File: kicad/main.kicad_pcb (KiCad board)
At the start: 2 copper layers, 119.4 x 99.1 mm, 41 parts, among them J1 Barrel_Jack, SW1 Reset, SW6 SW_DIP_x08, U1 KM1810VM88, U10 L7805, U11 15 MHz, U12 8255, U13 74HC273, U14 74HC244, U2 W27C512, U3 AS6C4008-55PCN, U4 74HC573, U5 74HC573, U6 ATF16V8, U7 DS1813-5+, U8 74HC00

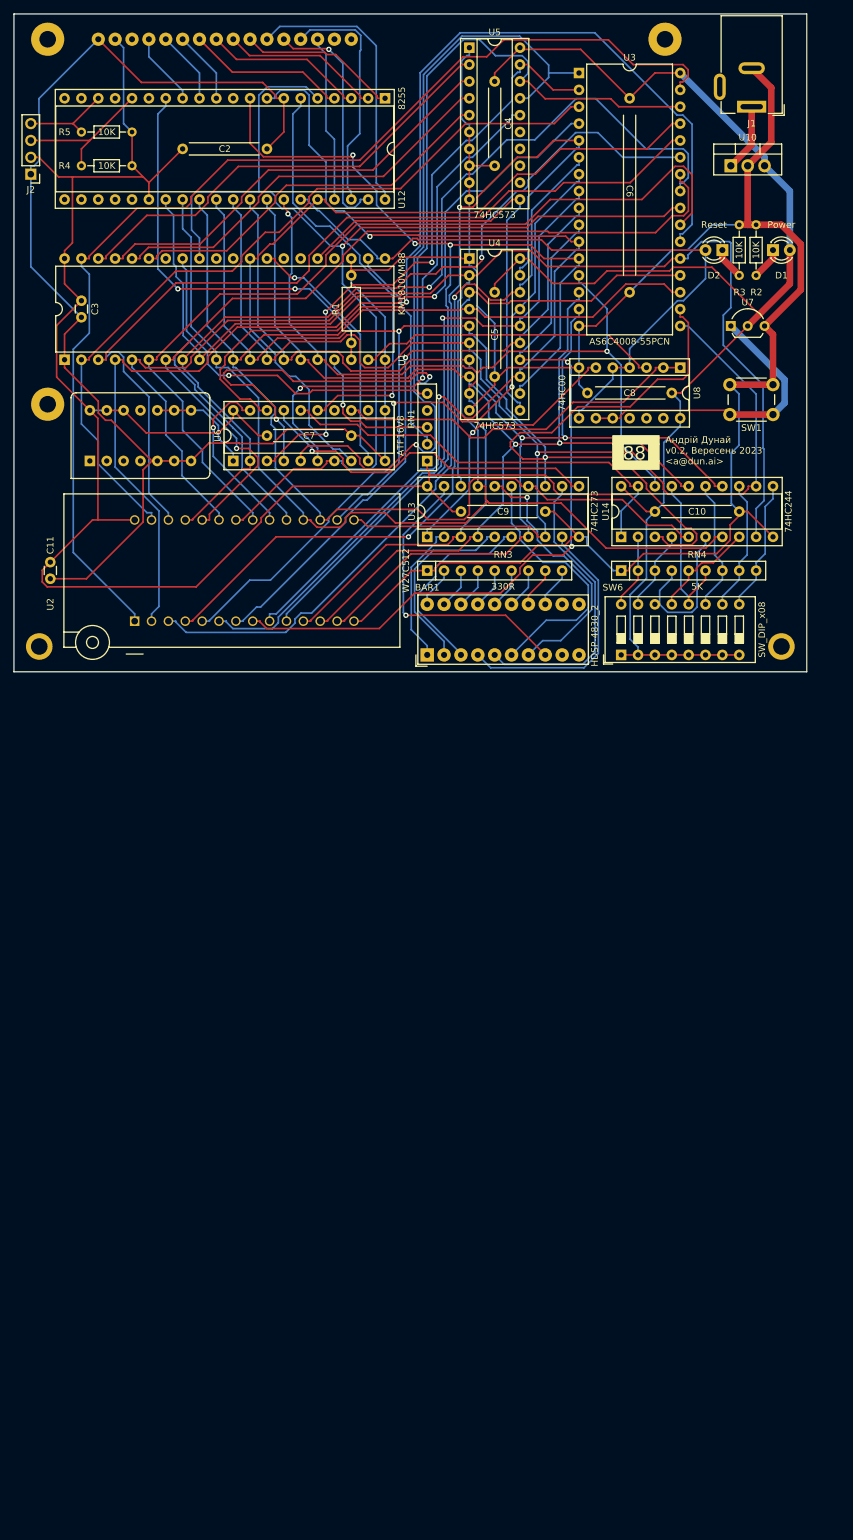
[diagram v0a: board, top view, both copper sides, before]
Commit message: Update PCB image
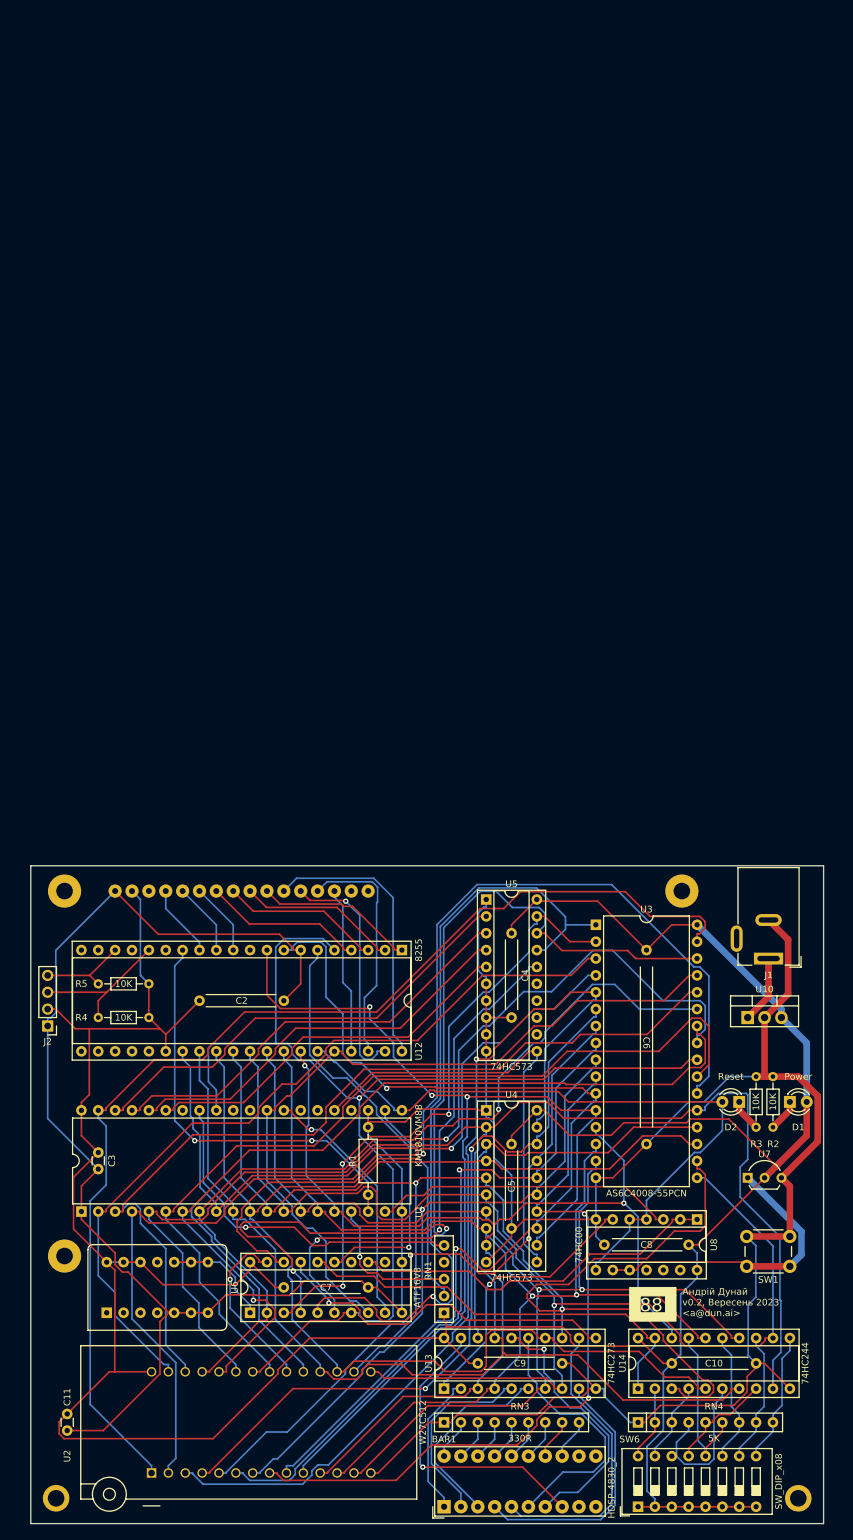
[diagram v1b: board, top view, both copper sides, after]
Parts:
- moved C10 128.3 mm to (114.3, 94.0)
- moved C2 128.3 mm to (43.2, 39.4)
- moved C3 128.3 mm to (27.9, 62.2)
- moved C4 128.3 mm to (90.2, 29.2)
- moved C5 128.3 mm to (90.2, 61.0)
- moved C6 128.3 mm to (110.5, 38.1)
- moved C8 128.3 mm to (116.8, 76.1)
- moved C9 128.3 mm to (85.1, 94.0)
- moved H1 128.3 mm to (21.6, 114.3)
- moved H2 128.3 mm to (133.3, 114.3)
- moved J1 128.3 mm to (128.9, 33.0)
- moved J2 128.3 mm to (20.3, 43.2)
- moved LCD1 128.3 mm to (20.3, 20.3)
- moved RN3 128.3 mm to (80.0, 102.9)
- moved RN4 128.3 mm to (109.2, 102.9)
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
